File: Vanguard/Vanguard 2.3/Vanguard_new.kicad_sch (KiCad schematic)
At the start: 84 parts, among them J1 USB_C_Receptacle_USB2.0_16P, J2 Conn_02x03_Pin, J3 Micro_SD_Card_Det1, J4 STARBOARD_SERVO, J5 PORTSIDE_SERVO, J6 Conn_01x02_Pin, J7 EJECTION_SERVO, Q1 BSS138, Q2 BSS138, Q3 BSS138, Q4 BSS138, U1 ATSAMD11D14A-M, U2 ATmega4809-A, U3 AT25DF641A-SH-T, U4 AP2112K-3.3, U5 BD1020HFV, U6 BNO086, U7 TXB0104D, U8 TPS61092, U9 MPM3610AGQV-P, Y1 32.768kHz

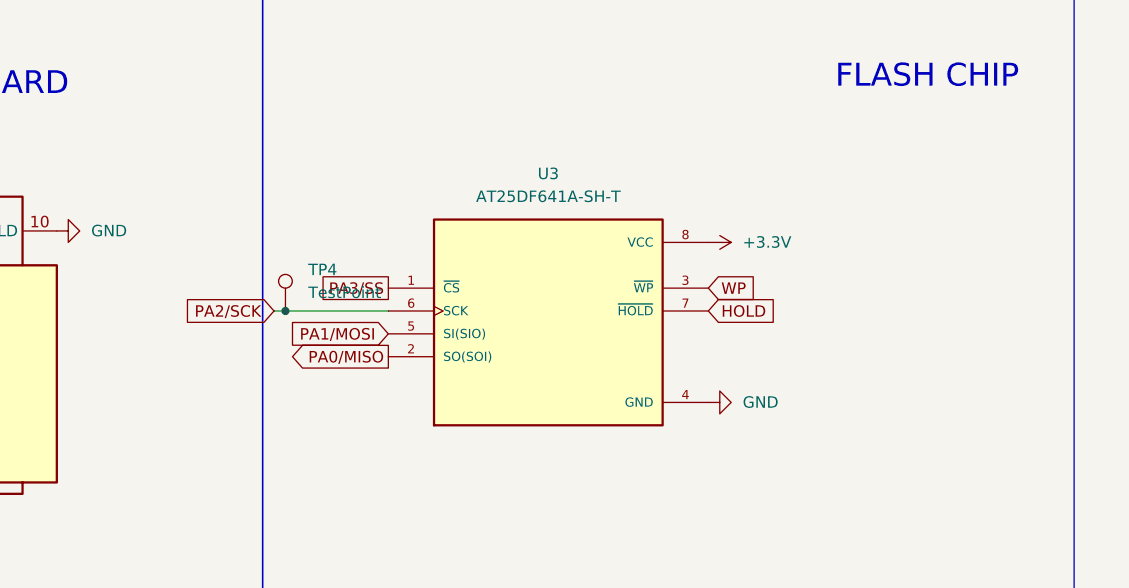
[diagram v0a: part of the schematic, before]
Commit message: kicad
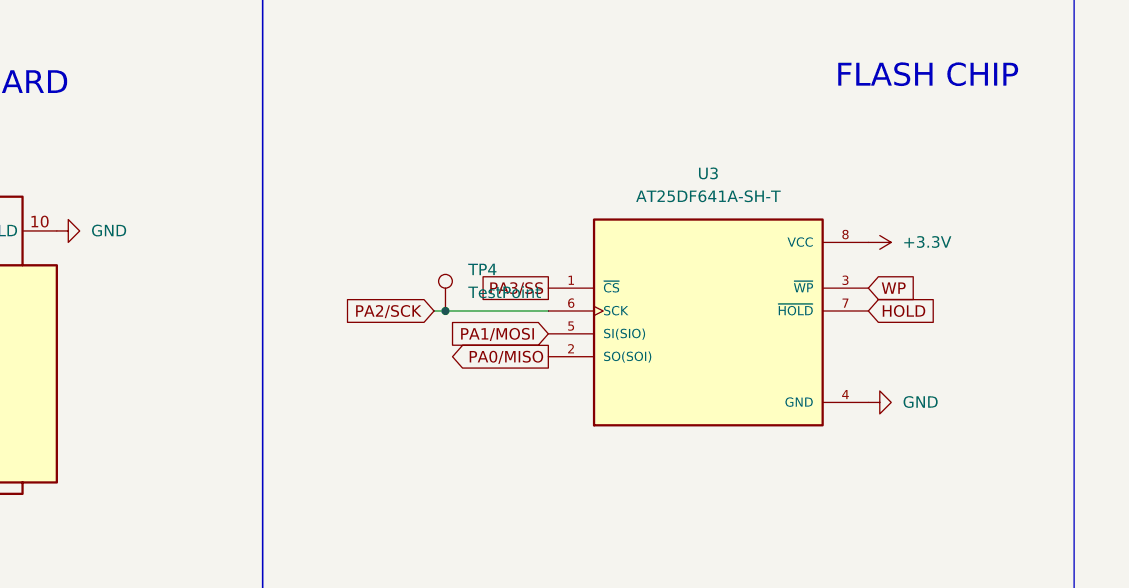
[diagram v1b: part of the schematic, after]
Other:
- moved on the sheet: TP4, U3
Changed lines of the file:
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@@
 	)
 	(junction
-		(at 140.97 231.14)
+		(at 158.75 231.14)
 		(diameter 0)
 		(color 0 0 0 0)
@@
 	(wire
 		(pts
-			(xy 140.97 231.14) (xy 152.4 231.14)
+			(xy 158.75 231.14) (xy 170.18 231.14)
 		)
 		(stroke
@@
 	(wire
 		(pts
-			(xy 139.7 231.14) (xy 140.97 231.14)
+			(xy 157.48 231.14) (xy 158.75 231.14)
 		)
 		(stroke
@@
 	(global_label "PA1{slash}MOSI"
 		(shape input)
-		(at 152.4 233.68 180)
+		(at 170.18 233.68 180)
 		(fields_autoplaced yes)
 		(effects
@@
 		)
 		(property "Intersheetrefs" "${INTERSHEET_REFS}"
-			(at 139.92 233.68 0)
+			(at 157.7 233.68 0)
 			(effects
 				(font
@@
 	(global_label "PA2{slash}SCK"
 		(shape input)
-		(at 139.7 231.14 180)
+		(at 157.48 231.14 180)
 		(fields_autoplaced yes)
 		(effects
@@
 		)
 		(property "Intersheetrefs" "${INTERSHEET_REFS}"
-			(at 128.0667 231.14 0)
+			(at 145.8467 231.14 0)
 			(effects
 				(font
@@
 	(global_label "PA0{slash}MISO"
 		(shape output)
-		(at 152.4 236.22 180)
+		(at 170.18 236.22 180)
 		(fields_autoplaced yes)
 		(effects
@@
 		)
 		(property "Intersheetrefs" "${INTERSHEET_REFS}"
-			(at 139.92 236.22 0)
+			(at 157.7 236.22 0)
 			(effects
 				(font
@@
 	(global_label "WP"
 		(shape input)
-		(at 187.96 228.6 0)
+		(at 205.74 228.6 0)
 		(fields_autoplaced yes)
 		(effects
@@
 		)
 		(property "Intersheetrefs" "${INTERSHEET_REFS}"
-			(at 193.6666 228.6 0)
+			(at 211.4466 228.6 0)
 			(effects
 				(font
@@
 	(global_label "PA3{slash}SS"
 		(shape passive)
-		(at 152.4 228.6 180)
+		(at 170.18 228.6 180)
 		(fields_autoplaced yes)
 		(effects
@@
 		)
 		(property "Intersheetrefs" "${INTERSHEET_REFS}"
-			(at 143.2085 228.6 0)
+			(at 160.9885 228.6 0)
 			(effects
 				(font
@@
 	(global_label "HOLD"
 		(shape input)
-		(at 187.96 231.14 0)
+		(at 205.74 231.14 0)
 		(fields_autoplaced yes)
 		(effects
@@
 		)
 		(property "Intersheetrefs" "${INTERSHEET_REFS}"
-			(at 195.9043 231.14 0)
+			(at 213.6843 231.14 0)
 			(effects
 				(font
@@
 	(symbol
 		(lib_id "Connector:TestPoint")
-		(at 140.97 231.14 0)
+		(at 158.75 231.14 0)
 		(unit 1)
 		(exclude_from_sim no)
@@
 		(fields_autoplaced yes)
 		(property "Reference" "TP4"
-			(at 143.51 226.5679 0)
+			(at 161.29 226.5679 0)
 			(effects
 				(font
@@
 		)
 		(property "Value" "TestPoint"
-			(at 143.51 229.1079 0)
+			(at 161.29 229.1079 0)
 			(effects
 				(font
@@
 		)
 		(property "Footprint" "TestPoint:TestPoint_Pad_1.0x1.0mm"
-			(at 146.05 231.14 0)
+			(at 163.83 231.14 0)
 			(effects
 				(font
@@
 		)
 		(property "Datasheet" "~"
-			(at 146.05 231.14 0)
+			(at 163.83 231.14 0)
 			(effects
 				(font
@@
 		)
 		(property "Description" "test point"
-			(at 140.97 231.14 0)
+			(at 158.75 231.14 0)
 			(effects
 				(font
@@
 	(symbol
 		(lib_id "power:+3.3V")
-		(at 187.96 223.52 270)
+		(at 205.74 223.52 270)
 		(unit 1)
 		(exclude_from_sim no)
@@
 		(fields_autoplaced yes)
 		(property "Reference" "#PWR052"
-			(at 184.15 223.52 0)
+			(at 201.93 223.52 0)
 			(effects
 				(font
@@
 		)
 		(property "Value" "+3.3V"
-			(at 191.77 223.5199 90)
+			(at 209.55 223.5199 90)
 			(effects
 				(font
@@
 		)
 		(property "Footprint" ""
-			(at 187.96 223.52 0)
+			(at 205.74 223.52 0)
 			(effects
 				(font
@@
 		)
 		(property "Datasheet" ""
-			(at 187.96 223.52 0)
+			(at 205.74 223.52 0)
 			(effects
 				(font
@@
 		)
 		(property "Description" "Power symbol creates a global label with name \"+3.3V\""
-			(at 187.96 223.52 0)
+			(at 205.74 223.52 0)
 			(effects
 				(font
@@
 	(symbol
 		(lib_id "AT25DF641A-SH-T:AT25DF641A-SH-T")
-		(at 170.18 233.68 0)
+		(at 187.96 233.68 0)
 		(unit 1)
 		(exclude_from_sim no)
@@
 		(fields_autoplaced yes)
 		(property "Reference" "U3"
-			(at 170.18 215.9 0)
+			(at 187.96 215.9 0)
 			(effects
 				(font
@@
 		)
 		(property "Value" "AT25DF641A-SH-T"
-			(at 170.18 218.44 0)
+			(at 187.96 218.44 0)
 			(effects
 				(font
@@
 		)
 		(property "Footprint" "Package_SO:SOIC-8_3.9x4.9mm_P1.27mm"
-			(at 170.18 233.68 0)
+			(at 187.96 233.68 0)
 			(effects
 				(font
@@
 		)
 		(property "Datasheet" ""
-			(at 170.18 233.68 0)
+			(at 187.96 233.68 0)
 			(effects
 				(font
@@
 		)
 		(property "Description" ""
-			(at 170.18 233.68 0)
+			(at 187.96 233.68 0)
 			(effects
 				(font
@@
 		)
 		(property "DigiKey_Part_Number" ""
-			(at 170.18 233.68 0)
+			(at 187.96 233.68 0)
 			(effects
 				(font
@@
 		)
 		(property "SnapEDA_Link" "https://www.snapeda.com/parts/AT25DF641A-SH-T/Dialog+Semiconductor/view-part/?ref=snap"
-			(at 170.18 233.68 0)
+			(at 187.96 233.68 0)
 			(effects
 				(font
@@
 		)
 		(property "MAXIMUM_PACKAGE_HEIGHT" "2.16 mm"
-			(at 170.18 233.68 0)
+			(at 187.96 233.68 0)
 			(effects
 				(font
@@
 		)
 		(property "Package" "SOIC-8 Dialog Semiconductor"
-			(at 170.18 233.68 0)
+			(at 187.96 233.68 0)
 			(effects
 				(font
@@
 		)
 		(property "Check_prices" "https://www.snapeda.com/parts/AT25DF641A-SH-T/Dialog+Semiconductor/view-part/?ref=eda"
-			(at 170.18 233.68 0)
+			(at 187.96 233.68 0)
 			(effects
 				(font
@@
 		)
 		(property "STANDARD" "IPC-7351B"
-			(at 170.18 233.68 0)
+			(at 187.96 233.68 0)
 			(effects
 				(font
@@
 		)
 		(property "PARTREV" "06-2020"
-			(at 170.18 233.68 0)
+			(at 187.96 233.68 0)
 			(effects
 				(font
@@
 		)
 		(property "MF" "Dialog Semiconductor"
-			(at 170.18 233.68 0)
+			(at 187.96 233.68 0)
 			(effects
 				(font
@@
 		)
 		(property "MP" "AT25DF641A-SH-T"
-			(at 170.18 233.68 0)
+			(at 187.96 233.68 0)
 			(effects
 				(font
@@
 		)
 		(property "Description_1" "\n64 Mbit, 3.0V (2.7V to 3.6V), -40C to 85C, SOIC-W 208mil (Tape & Reel), Single, Dual SPI NOR flash\n"
-			(at 170.18 233.68 0)
+			(at 187.96 233.68 0)
 			(effects
 				(font
@@
 		)
 		(property "MANUFACTURER" "Dialog Semiconductor"
-			(at 170.18 233.68 0)
+			(at 187.96 233.68 0)
 			(effects
 				(font
@@
 	(symbol
 		(lib_id "power:GND")
-		(at 187.96 241.3 90)
+		(at 205.74 241.3 90)
 		(unit 1)
 		(exclude_from_sim no)
@@
 		(fields_autoplaced yes)
 		(property "Reference" "#PWR053"
-			(at 194.31 241.3 0)
+			(at 212.09 241.3 0)
 			(effects
 				(font
@@
 		)
 		(property "Value" "GND"
-			(at 191.77 241.2999 90)
+			(at 209.55 241.2999 90)
 			(effects
 				(font
@@
 		)
 		(property "Footprint" ""
-			(at 187.96 241.3 0)
+			(at 205.74 241.3 0)
 			(effects
 				(font
@@
 		)
 		(property "Datasheet" ""
-			(at 187.96 241.3 0)
+			(at 205.74 241.3 0)
 			(effects
 				(font
@@
 		)
 		(property "Description" "Power symbol creates a global label with name \"GND\" , ground"
-			(at 187.96 241.3 0)
+			(at 205.74 241.3 0)
 			(effects
 				(font
